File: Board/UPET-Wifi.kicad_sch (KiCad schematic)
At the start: 17 parts, among them J1 Conn_01x03_Pin, J2 Conn_01x05_Pin, U1 ESP32-C3-WROOM-02, U2 SC16IS752IPW, U3 1.8432 MHz

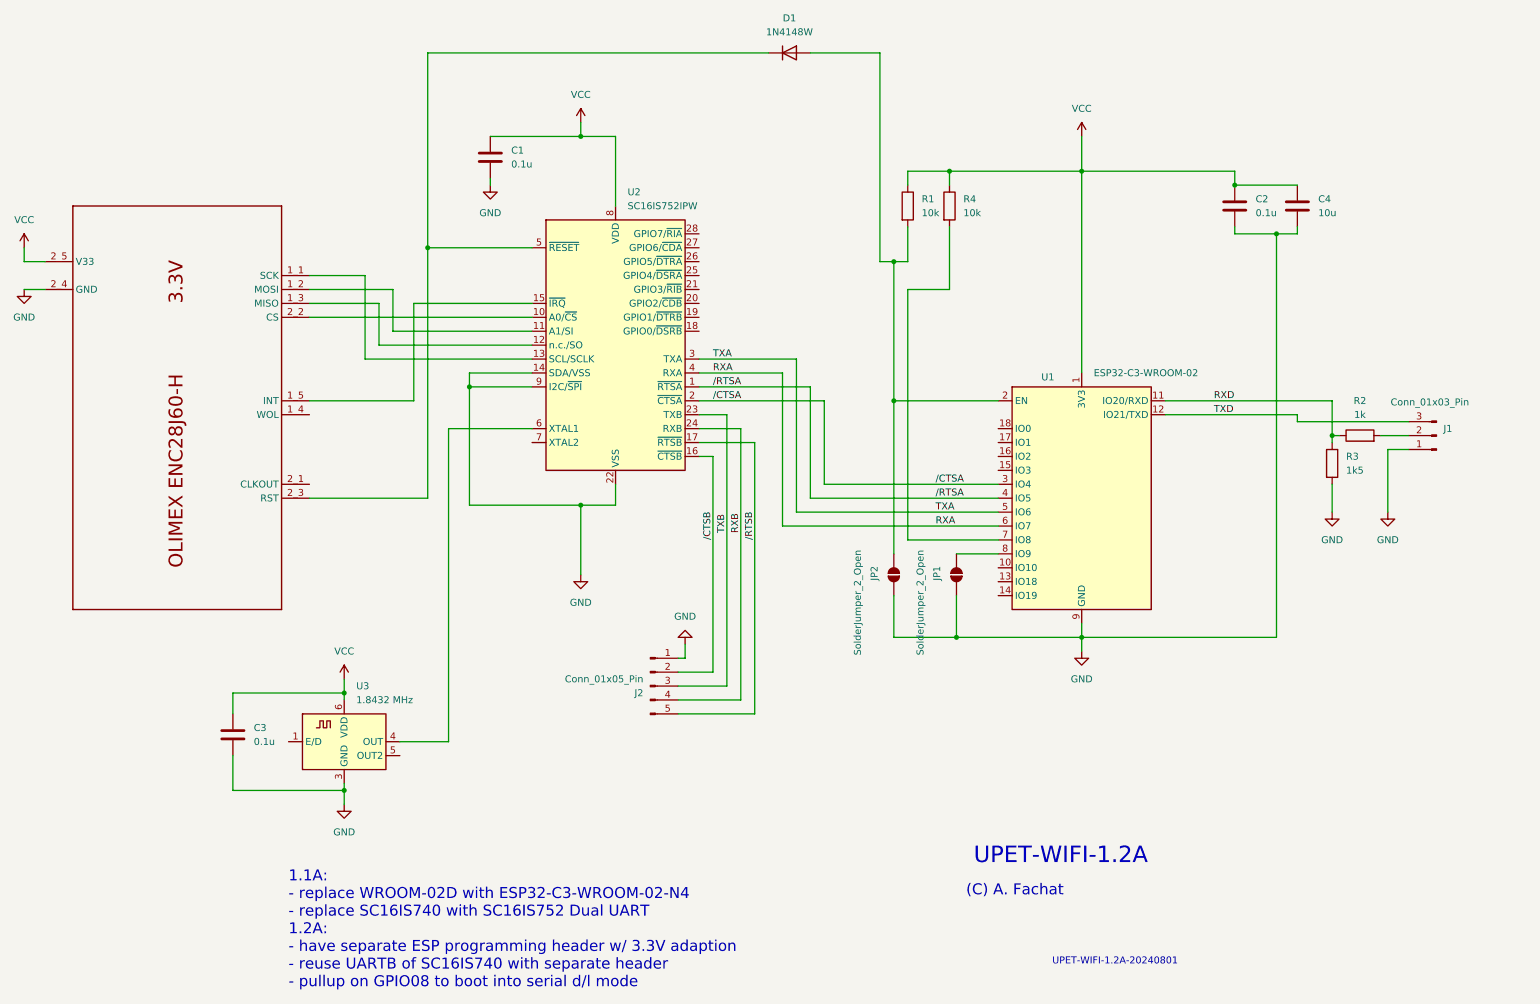
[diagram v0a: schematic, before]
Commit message: work on wifi 1.3a
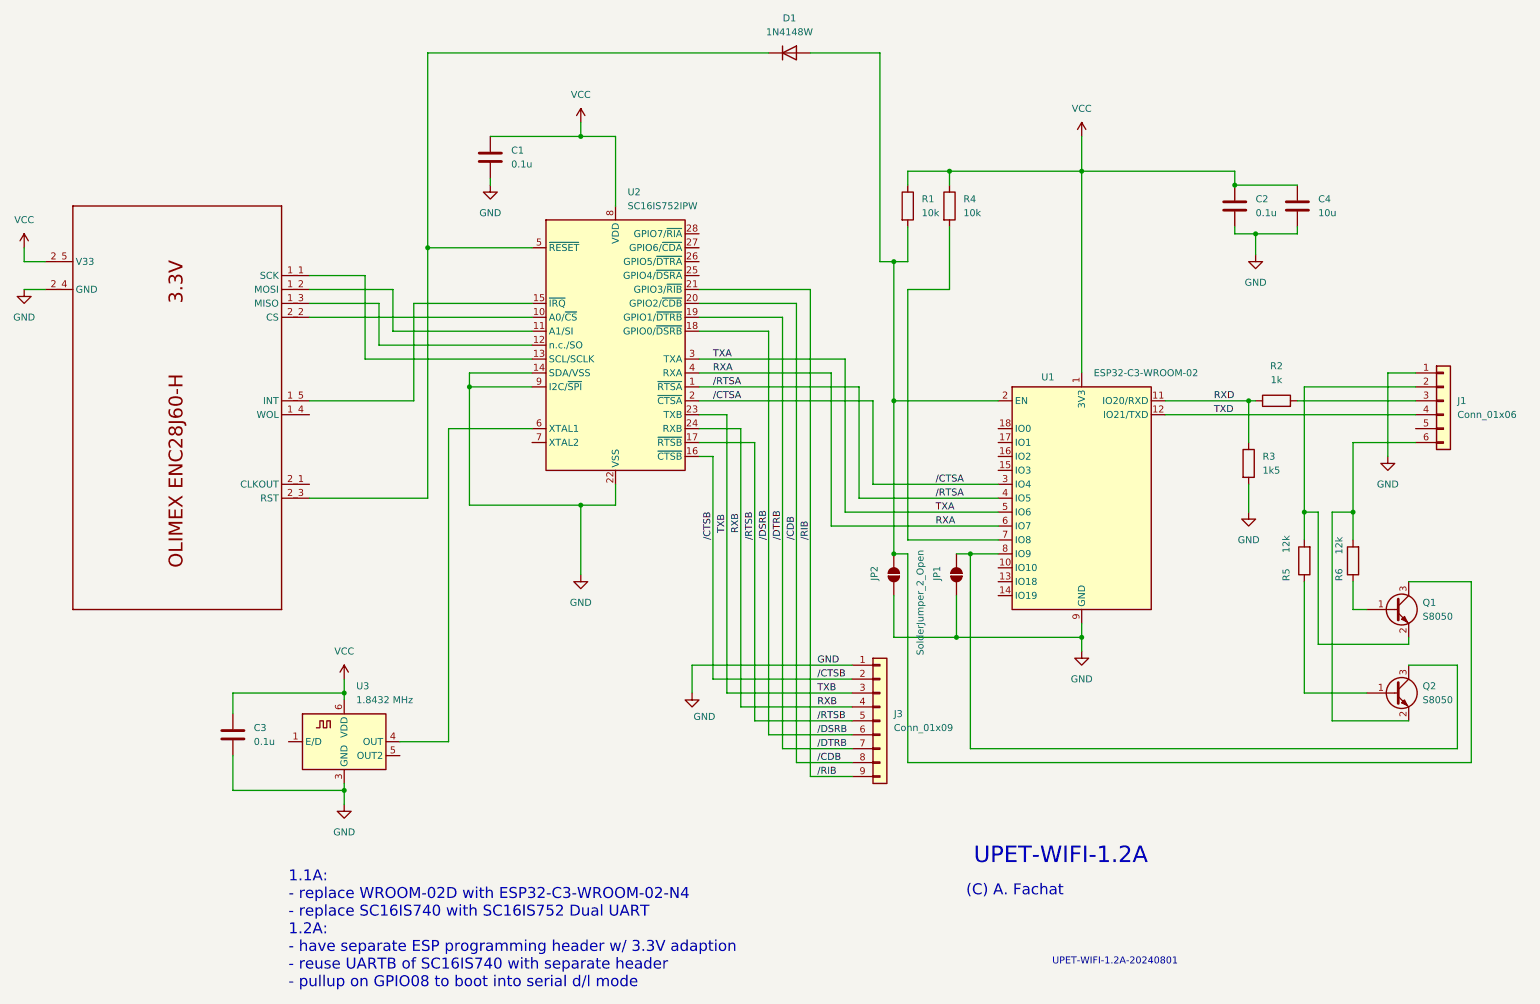
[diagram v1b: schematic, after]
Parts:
- removed J1: Conn_01x03_Pin, Connector_PinHeader_2.54mm:PinHeader_1x03_P2.54mm_Vertical, symbol Connector:Conn_01x03_Pin
- removed J2: Conn_01x05_Pin, Connector_PinHeader_2.54mm:PinHeader_1x05_P2.54mm_Vertical, symbol Connector:Conn_01x05_Pin
- added J1: Conn_01x06, Connector_PinHeader_2.54mm:PinHeader_1x06_P2.54mm_Vertical, symbol Connector_Generic:Conn_01x06
- added J3: Conn_01x09, Connector_PinHeader_2.54mm:PinHeader_1x09_P2.54mm_Vertical, symbol Connector_Generic:Conn_01x09
- added Q1, Q2: S8050, Package_TO_SOT_SMD:SOT-23, symbol Transistor_BJT:S8050
- added R5, R6: 12k, Resistor_SMD:R_0603_1608Metric_Pad0.98x0.95mm_HandSolder, symbol Device:R
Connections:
- net GND: now also J1.1 (Pin_1), J3.1 (Pin_1)
- net RXB: now also J3.4 (Pin_4)
- net TXB: now also J3.3 (Pin_3)
- net TXD: now also J1.4 (Pin_4)
- net /CTSB: now also J3.2 (Pin_2)
- net /RTSB: now also J3.5 (Pin_5)
- net at D1.2 (A), JP2.2 (B), R1.2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: now also Q1.3 (C)
- net at JP1.2 (B), U1.8 (IO9): now also Q2.3 (C)
- net at R2.2: now also J1.3 (Pin_3)
- net /DSRB: now reaches U2.18 (GPIO0/~{DSRB})
- net /DSRB: now also J3.6 (Pin_6)
- net /DTRB: now reaches U2.19 (GPIO1/~{DTRB})
- net /DTRB: now also J3.7 (Pin_7)
- net /CDB: now reaches U2.20 (GPIO2/~{CDB})
- net /CDB: now also J3.8 (Pin_8)
- net /RIB: now reaches U2.21 (GPIO3/~{RIB})
- net /RIB: now also J3.9 (Pin_9)
- new net: Q2.1 (B), R5.1
- new net: J1.6 (Pin_6), Q2.2 (E), R6.2
- new net: J1.2 (Pin_2), Q1.2 (E), R5.2
- new net: Q1.1 (B), R6.1
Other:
- moved on the sheet: R2, R3
